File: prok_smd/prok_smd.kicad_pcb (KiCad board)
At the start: 2 copper layers, 105 x 41.2 mm, 60 parts, among them CON1 microSD_Card, J1 POWER, J10 Conn_01x02_Female, J11 Conn_01x02_Female, J12 Conn_01x05_Male, J13 Conn_01x02_Female, J14 Conn_01x02_Female, J15 Conn_01x02_Male, J16 Conn_01x02_Male, J17 Conn_01x02_Male, J18 Conn_01x02_Male, J5 TIME_CV, J6 CHANNEL_CV, J7 RESET_CV, J8 OUT, J9 Conn_01x05_Female, SW1 SW_Push_LED, U1 Teensy3.2, U2 MCP6002, U3 TL072, U4 REG1117

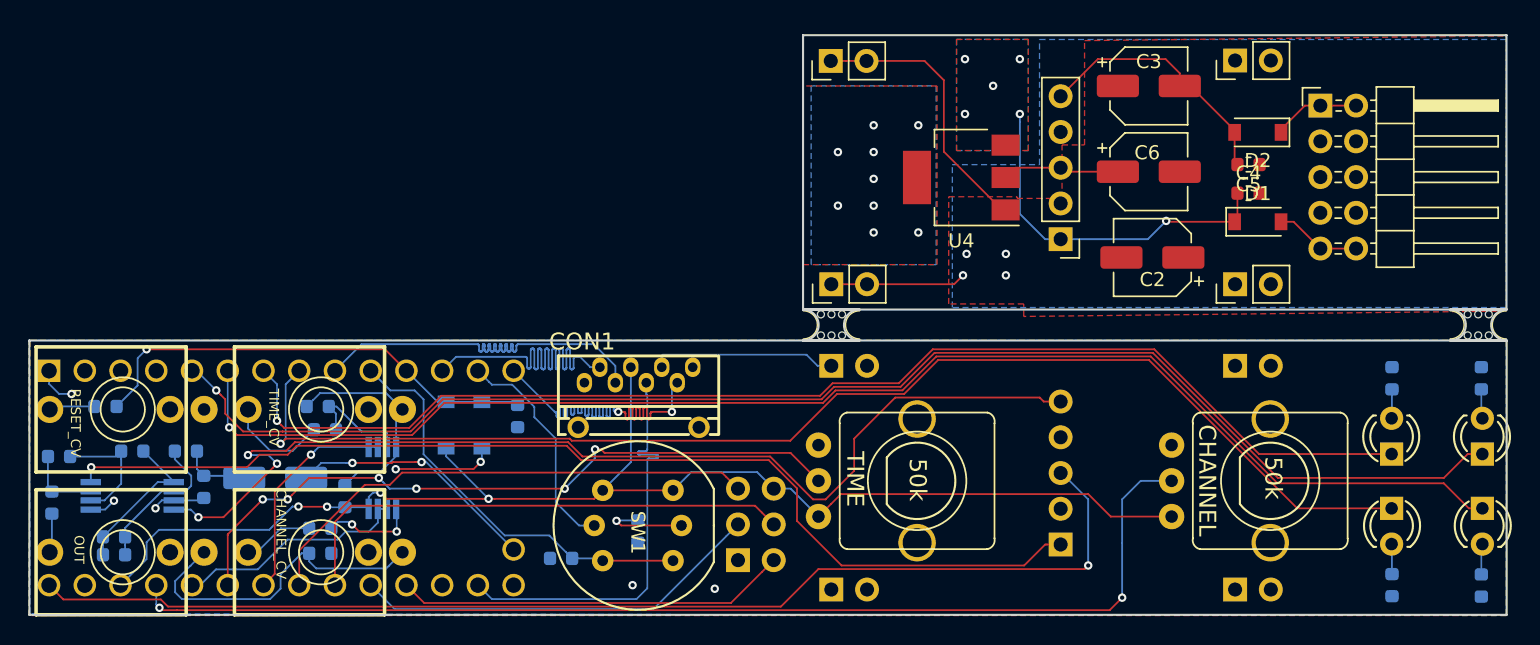
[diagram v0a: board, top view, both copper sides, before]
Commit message: :sparkles: :construction: first draft v2 board
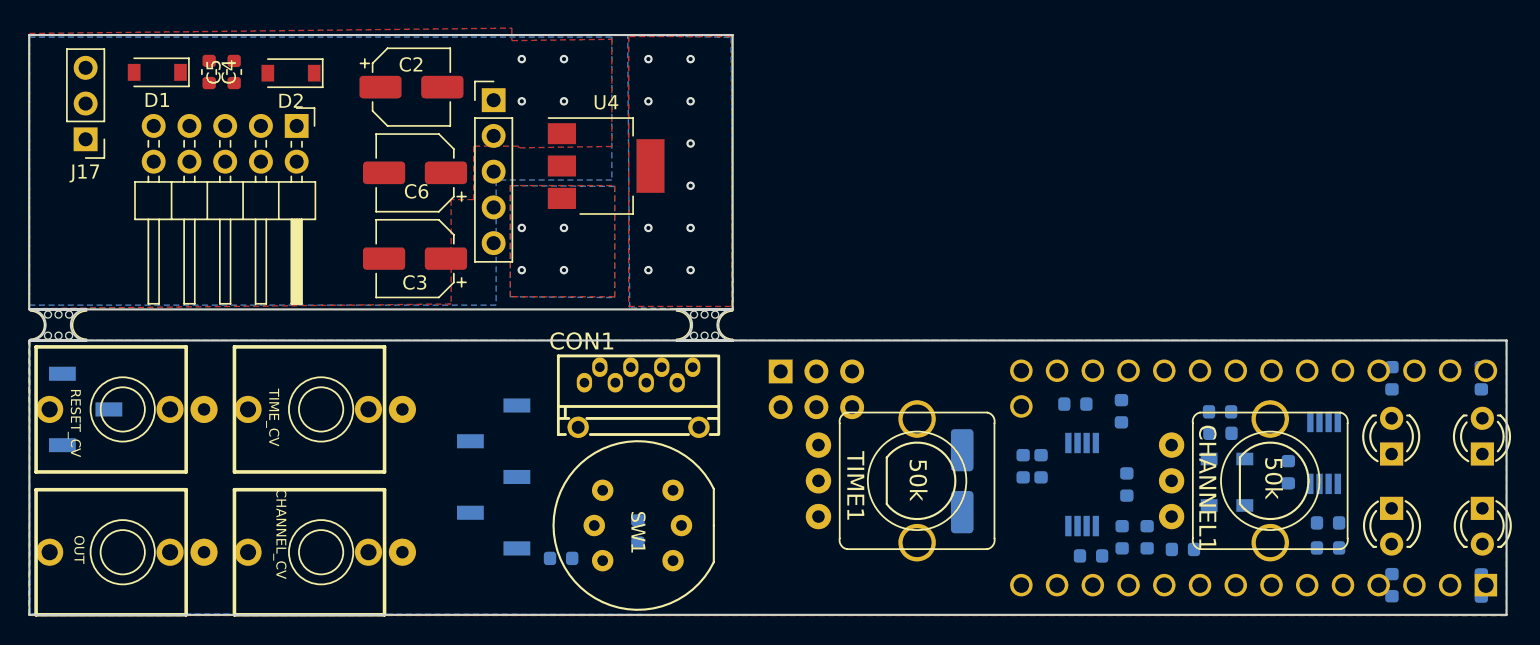
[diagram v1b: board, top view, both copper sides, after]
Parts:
- removed J10, J11, J13, J14: Conn_01x02_Female, Connector_PinSocket_2.54mm:PinSocket_1x02_P2.54mm_Vertical
- removed J15, J16, J18: Conn_01x02_Male, Connector_PinHeader_2.54mm:PinHeader_1x02_P2.54mm_Vertical
- added J2: Conn_01x03_Female, Connector_PinSocket_2.54mm:PinSocket_1x03_P2.54mm_Vertical_SMD_Pin1Left, B.Cu at (104.0, 59.9)
- J17: value Conn_01x02_Male -> Conn_01x03_Male; footprint Connector_PinHeader_2.54mm:PinHeader_1x02_P2.54mm_Vertical -> Connector_PinHeader_2.54mm:PinHeader_1x03_P2.54mm_Vertical
- J9: footprint Connector_PinSocket_2.54mm:PinSocket_1x05_P2.54mm_Vertical -> Connector_PinSocket_2.54mm:PinSocket_1x05_P2.54mm_Vertical_SMD_Pin1Left
- moved mouse-bite-2mm-slot 100.9 mm to (102.1, 53.9), turned to 180 degrees
- moved J17 81.9 mm to (104.0, 40.7), turned to 180 degrees
- moved D1 78.9 mm to (109.1, 35.9), turned to 180 degrees
- moved R5 75.6 mm to (177.6, 60.0), turned to 270 degrees
- moved R10 74.6 mm to (179.5, 69.0), turned to 90 degrees
- moved C4 74.4 mm to (112.8, 35.9), turned to 270 degrees
- moved R18 73.1 mm to (174.3, 59.5), turned to 180 degrees
- moved J1 72.8 mm to (119.0, 39.8), turned to 270 degrees
- moved C5 72.4 mm to (114.6, 35.9), turned to 90 degrees
- moved R7 71.6 mm to (192.3, 68.0)
- moved R9 71.6 mm to (192.3, 69.7)
- moved R4 70.7 mm to (178.0, 65.2), turned to 270 degrees
- moved D2 68.8 mm to (118.6, 36.0)
- moved U1 68.7 mm to (186.8, 64.8), turned to 180 degrees
- moved U3 67.5 mm to (174.8, 65.2), turned to 90 degrees
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- renumbered CHANNEL to CHANNEL1, EXPAND to EXPAND1, TIME to TIME1
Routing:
- net +12V: track 101.9 -> 0.00 mm, vias 7 -> 4
- net LED_1: track 100.8 -> 0.00 mm, vias 1 -> 0
- net LED_2: track 100.2 -> 0.00 mm, vias 1 -> 0
- net GND: track 97.4 -> 0.00 mm, vias 11 -> 4
- net +3V3: track 96.9 -> 0.00 mm, vias 4 -> 0
- net -12V: track 94.3 -> 0.00 mm, vias 3 -> 0
- net LED_4: track 91.7 -> 0.00 mm, vias 1 -> 0
- net +5V: track 91.6 -> 0.00 mm, vias 1 -> 0
- net LED_3: track 88.9 -> 0.00 mm, vias 1 -> 0
- net CHANNEL_POT: track 81.6 -> 0.00 mm, vias 2 -> 0
- net TIME_POT: track 50.0 -> 0.00 mm, vias 6 -> 0
- net A4: track 36.7 -> 0.00 mm
- net A5: track 36.4 -> 0.00 mm
- net RESET_CV: track 33.0 -> 0.00 mm, vias 1 -> 0
- net MISO: track 30.0 -> 0.00 mm, vias 2 -> 0
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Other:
- outline, holes or cut-outs redrawn

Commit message: :sparkles: :construction: first draft routing v2
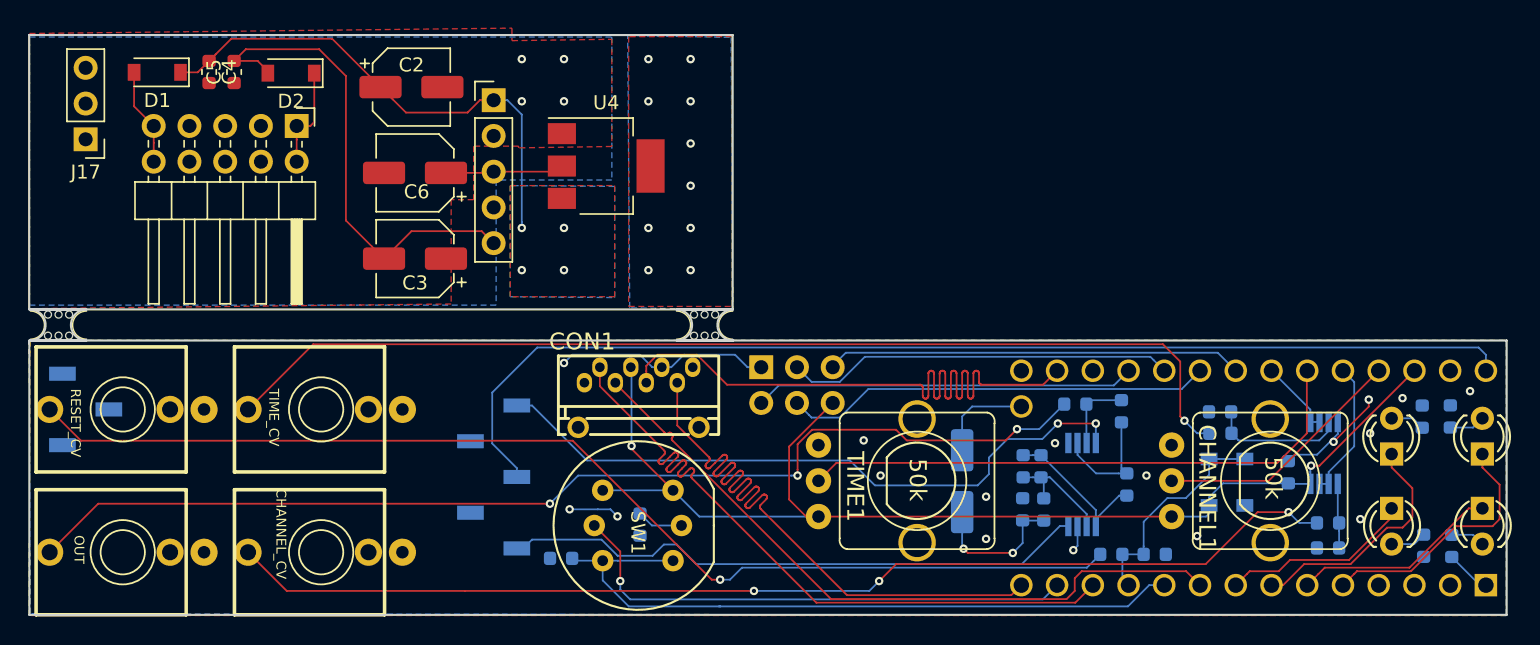
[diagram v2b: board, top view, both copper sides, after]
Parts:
- moved R2 5.91 mm to (172.1, 67.0)
- moved R1 5.88 mm to (170.6, 67.0), turned to 270 degrees
- moved R16 3.59 mm to (199.1, 69.6)
- moved R14 3.51 mm to (201.1, 69.6)
- moved R13 3.50 mm to (201.0, 60.4)
- moved R15 3.47 mm to (199.0, 60.4)
- moved R10 2.82 mm to (176.9, 70.2), turned to 180 degrees
- moved R11 2.03 mm to (180.0, 70.2)
- moved EXPAND1 1.41 mm to (152.0, 56.9)
- moved R17 0.51 mm to (143.4, 68.1)
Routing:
- net +5V: track 0.00 -> 88.5 mm
- net +3V3: track 0.00 -> 85.1 mm, vias 0 -> 2
- net +12V: track 0.00 -> 83.7 mm, vias 4 -> 6
- net Net-(J7-PadT): track 0.00 -> 80.4 mm, vias 0 -> 1
- net Net-(J6-PadT): track 0.00 -> 79.8 mm, vias 0 -> 3
- net Net-(J8-PadT): track 0.00 -> 78.4 mm, vias 0 -> 3
- net -12V: track 0.00 -> 76.9 mm
- net Net-(J5-PadT): track 0.00 -> 75.2 mm, vias 0 -> 1
- net MOSI: track 0.00 -> 50.1 mm
- net RESET_SW: track 0.00 -> 50.0 mm
- net MISO: track 0.00 -> 50.0 mm
- net SCLK: track 0.00 -> 50.0 mm
- net SS: track 0.00 -> 50.0 mm
- net TIME_POT: track 0.00 -> 40.6 mm
- net LED_RESET: track 0.00 -> 37.1 mm, vias 0 -> 1
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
